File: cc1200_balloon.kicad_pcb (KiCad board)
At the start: 4 copper layers, 50 x 30 mm, 107 parts, among them J101 BATT pads, J201 LoRa ANT pads, J202 SWD+DBG pads, J301 434MHz ANT pads, J401 GNSS ANT, J501 BMV080, Q101 DMG3401LSN-7, U201 Wio-E5, U301 CC1200, U401 AT6558R-5N32, U501 SCD40-D-R2, U502 AS3935-BQFT, U503 BME688, U504 BME688, X301 40MHz, X401 TCXO 26MHz, X402 32.768kHz

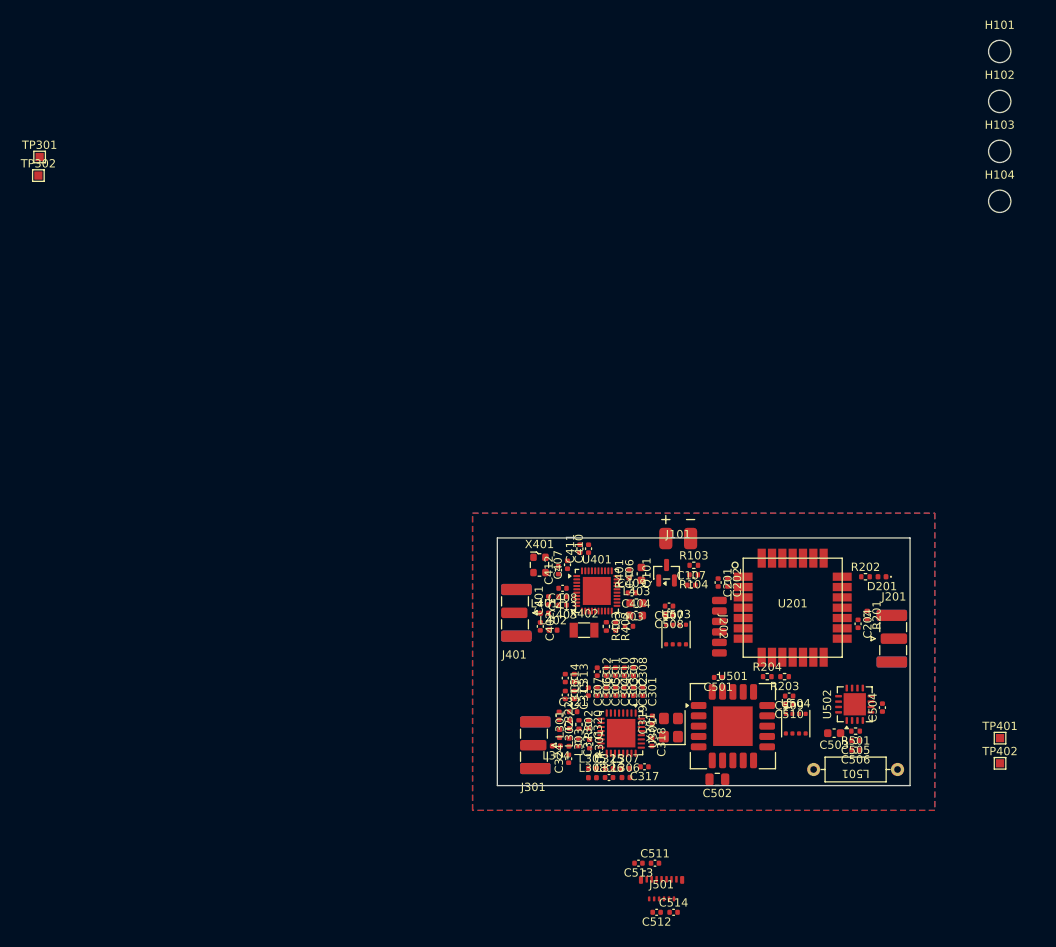
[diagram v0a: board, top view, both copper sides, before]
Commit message: Inital routing
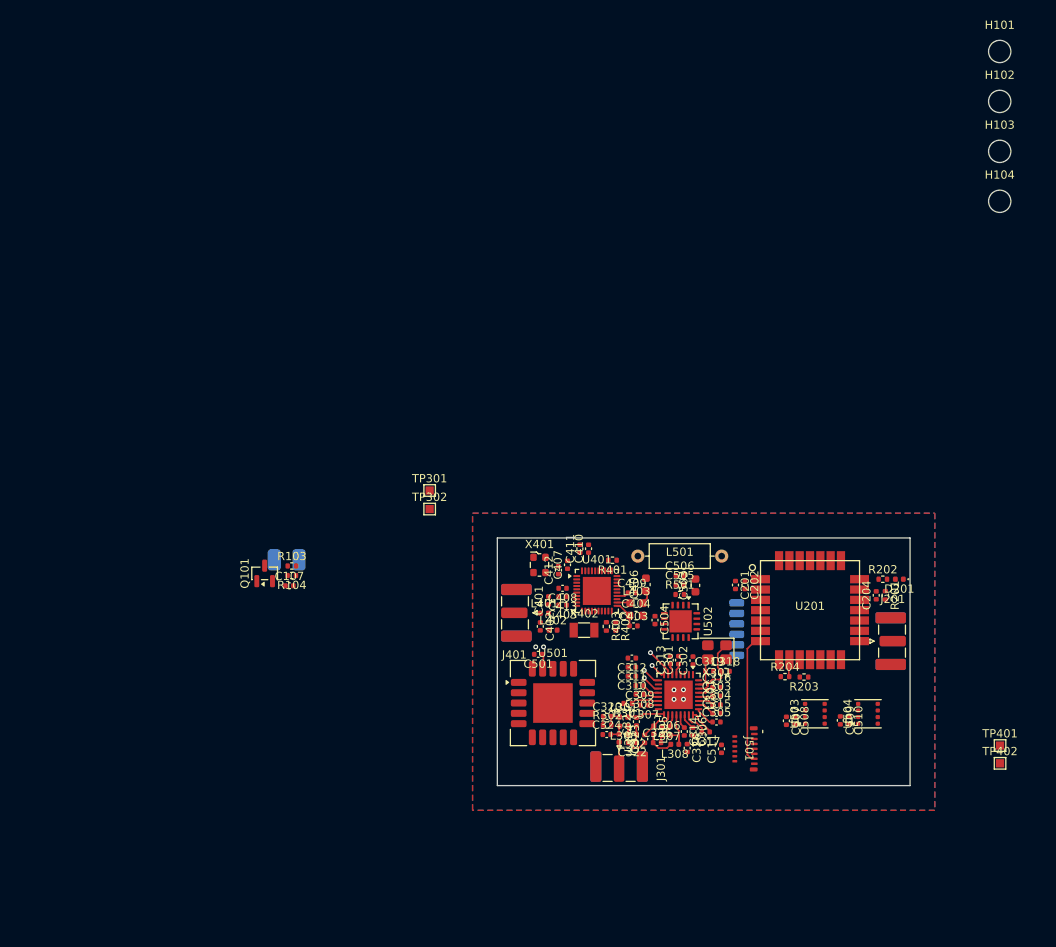
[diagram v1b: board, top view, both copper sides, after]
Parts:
- removed C502: 22u, Capacitor_SMD:C_0805_2012Metric
- removed C512, C513: 1u, Capacitor_SMD:C_0402_1005Metric
- removed C514: 100n, Capacitor_SMD:C_0402_1005Metric
- J101, J202: moved to B.Cu
- moved TP302 62.3 mm to (66.8, 81.5)
- moved TP301 62.2 mm to (66.8, 79.2)
- moved R104 48.7 mm to (50.1, 89.5)
- moved C107 48.7 mm to (49.8, 90.8)
- moved Q101 48.7 mm to (46.8, 89.3)
- moved R103 48.7 mm to (50.1, 88.4)
- moved J101 47.5 mm to (49.5, 87.7), turned to 180 degrees
- moved L501 33.5 mm to (97.1, 87.2), turned to 0 degrees
- moved C506 30.0 mm to (97.1, 89.5), turned to 0 degrees
- moved C504 29.5 mm to (94.1, 95.0), turned to -90 degrees
- moved C505 28.4 mm to (97.1, 90.7), turned to 0 degrees
- moved R501 27.0 mm to (97.1, 91.8), turned to 0 degrees
- moved C503 24.5 mm to (99.0, 90.8), turned to 90 degrees
- moved U502 23.4 mm to (97.2, 95.1), turned to -90 degrees
- moved C501 22.0 mm to (80.0, 99.1)
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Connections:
- U501 pad 10: SCL -> SDA
- U501 pad 9: SDA -> SCL
- U502 pad 11: SDA -> SCL
- U502 pad 13: SCL -> SDA
- U503 pad 3: SCL -> SDA
- U503 pad 4: SDA -> SCL
- U504 pad 3: SCL -> SDA
- U504 pad 4: SDA -> SCL
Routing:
- net +BATT: track 0.00 -> 21.0 mm, vias 0 -> 1
- net SPI_MISO: track 0.00 -> 18.1 mm, vias 0 -> 1
- net /CC1200 Radio/XOSC_Q1: track 0.00 -> 8.01 mm
- net /CC1200 Radio/RF_LNAN: track 0.00 -> 5.81 mm
- net /CC1200 Radio/RF_TX2: track 0.00 -> 4.57 mm
- net /CC1200 Radio/RF_PA: track 0.00 -> 4.37 mm
- net /CC1200 Radio/RF_TRXSW: track 0.00 -> 4.16 mm
- net /CC1200 Radio/RF_LNAP: track 0.00 -> 3.93 mm
- net /CC1200 Radio/XOSC_Q2: track 0.00 -> 3.80 mm
- net /CC1200 Radio/RF_RX1: track 0.00 -> 3.70 mm
- net SPI_MOSI: track 0.00 -> 3.55 mm, vias 0 -> 1
- net /CC1200 Radio/CC_RBIAS: track 0.00 -> 3.42 mm
- net Net-(U301-LPF1): track 0.00 -> 3.13 mm
- net Net-(U301-LPF0): track 0.00 -> 3.03 mm
- net RADIO_CS: track 0.00 -> 2.28 mm, vias 0 -> 1
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
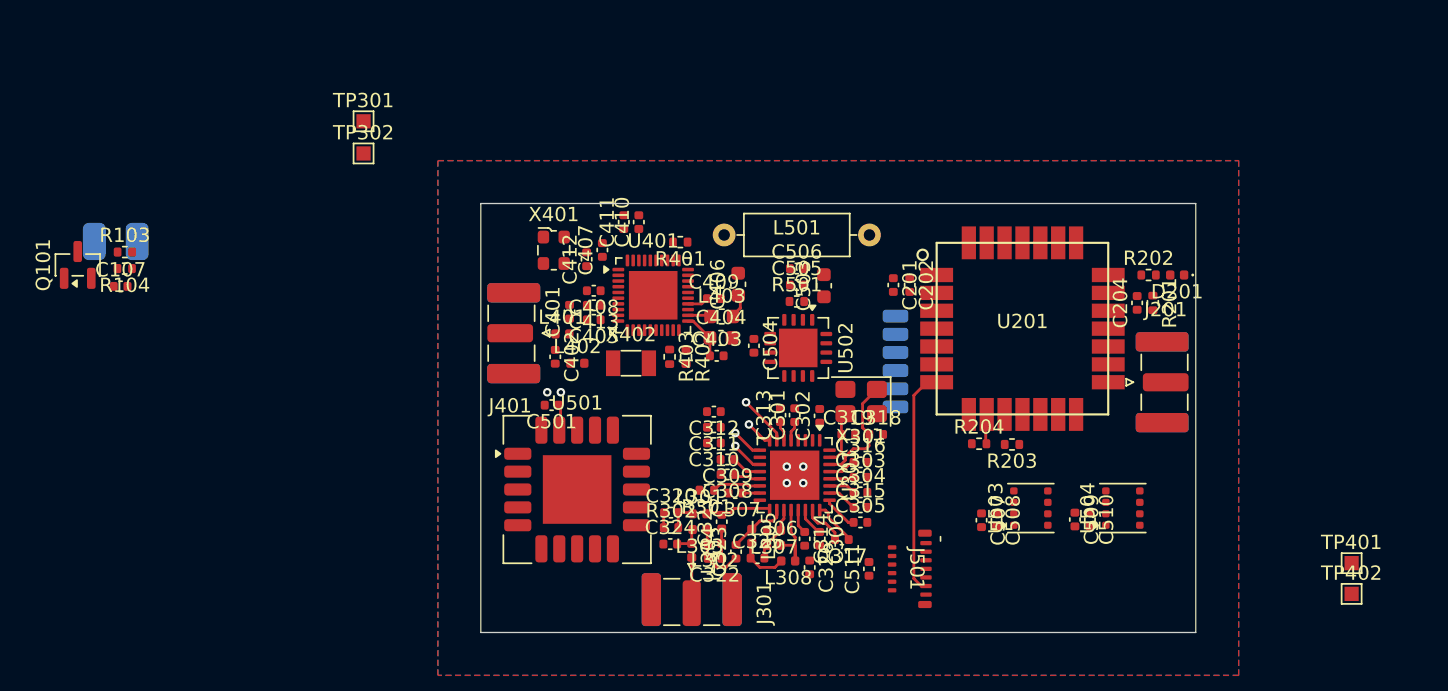
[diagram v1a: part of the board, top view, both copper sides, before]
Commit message: More routing.
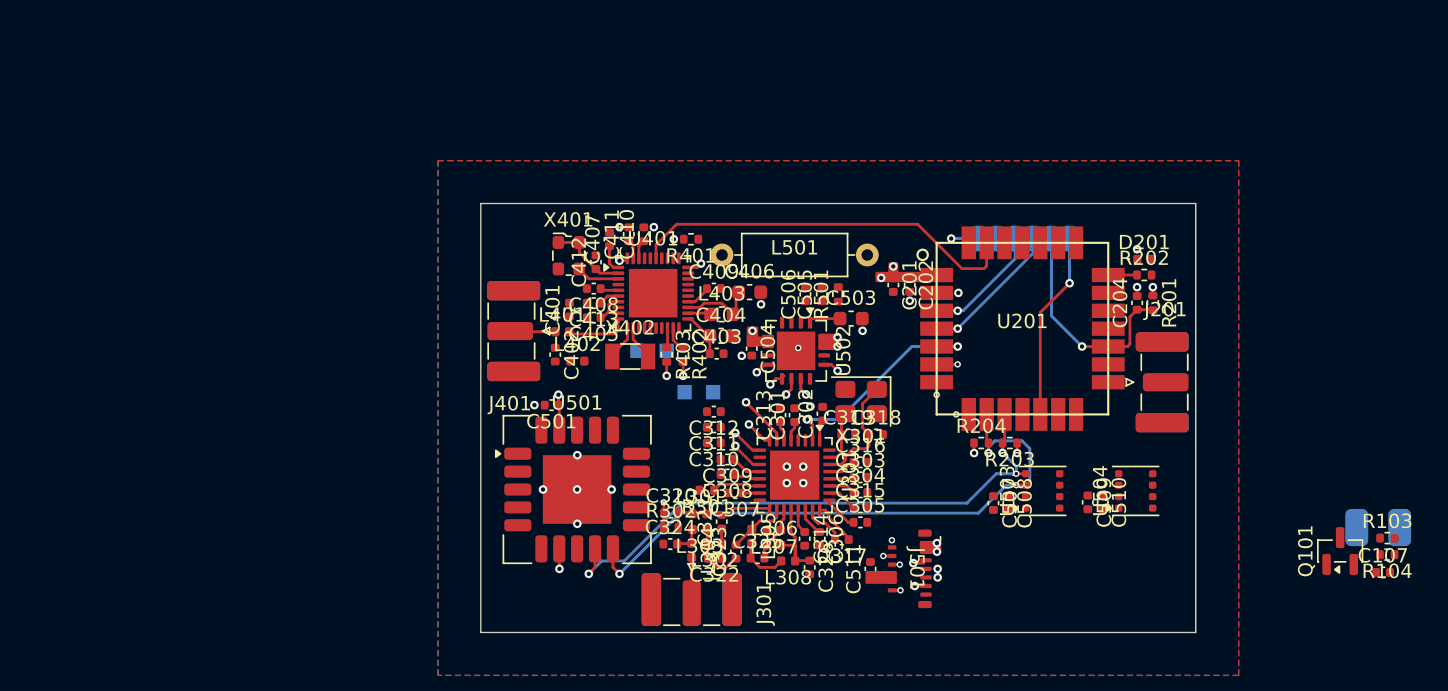
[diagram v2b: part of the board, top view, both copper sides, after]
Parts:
- TP301, TP302, TP401, TP402: moved to B.Cu
- moved R103 90.5 mm to (138.4, 108.4)
- moved C107 90.5 mm to (138.1, 110.8)
- moved J101 90.5 mm to (137.8, 107.7)
- moved Q101 90.5 mm to (135.1, 109.3)
- moved R104 90.5 mm to (138.4, 109.6)
- moved TP401 52.1 mm to (86.0, 95.3), turned to 180 degrees
- moved TP402 50.8 mm to (88.0, 95.3), turned to 180 degrees
- moved TP302 29.6 mm to (91.2, 98.2), turned to -90 degrees
- moved TP301 29.4 mm to (89.2, 98.2), turned to -90 degrees
- moved J202 12.4 mm to (113.0, 87.5), turned to 0 degrees
- moved C503 2.98 mm to (100.9, 93.0), turned to 0 degrees
- moved R501 2.94 mm to (100.0, 91.3), turned to 90 degrees
- moved D201 2.55 mm to (121.4, 88.9), turned to 0 degrees
- moved C506 1.90 mm to (97.7, 91.3), turned to 90 degrees
- moved C505 1.87 mm to (98.8, 91.3), turned to 90 degrees
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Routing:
- net SDA: track 2.08 -> 43.9 mm, vias 0 -> 4
- net SCL: track 0.00 -> 41.2 mm, vias 0 -> 4
- net GNSS_PPS: track 0.00 -> 27.6 mm
- net RADIO_RST: track 0.00 -> 15.8 mm, vias 0 -> 2
- net NRST: track 0.00 -> 15.6 mm, vias 0 -> 1
- net SPI_MISO: track 18.1 -> 3.87 mm, vias 1 -> 3
- net /MCU/DBG_TX: track 0.00 -> 13.1 mm, vias 0 -> 1
- net +BATT: track 21.0 -> 33.3 mm, vias 1 -> 16
- net /MCU/SWCLK: track 0.00 -> 9.96 mm, vias 0 -> 1
- net /MCU/SWDIO: track 0.00 -> 8.41 mm, vias 0 -> 1
- net /GNSS/GNSS_VX: track 0.00 -> 5.48 mm
- net /GNSS/GNSS_ANT_BIAS: track 0.00 -> 4.16 mm
- net /GNSS/GNSS_VCORE: track 1.75 -> 5.30 mm
- net /GNSS/GNSS_XREF: track 0.00 -> 3.03 mm
- net /GNSS/GNSS_RTC_O: track 0.00 -> 2.43 mm
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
